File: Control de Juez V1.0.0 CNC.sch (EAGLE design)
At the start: 21 parts, among them Q1 MMBT3904, U1 ATTINY412-SSNSOIC8_SA_SST_MCH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

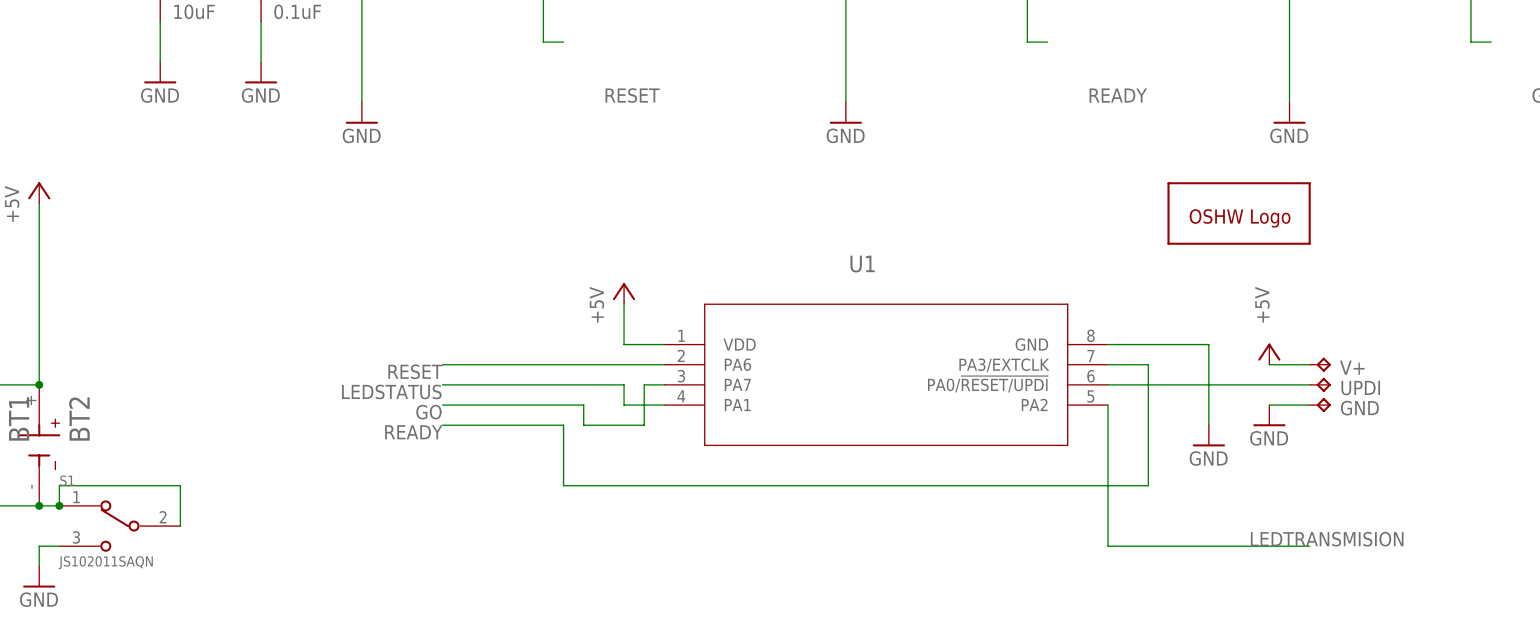
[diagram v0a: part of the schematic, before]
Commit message: Add files via upload
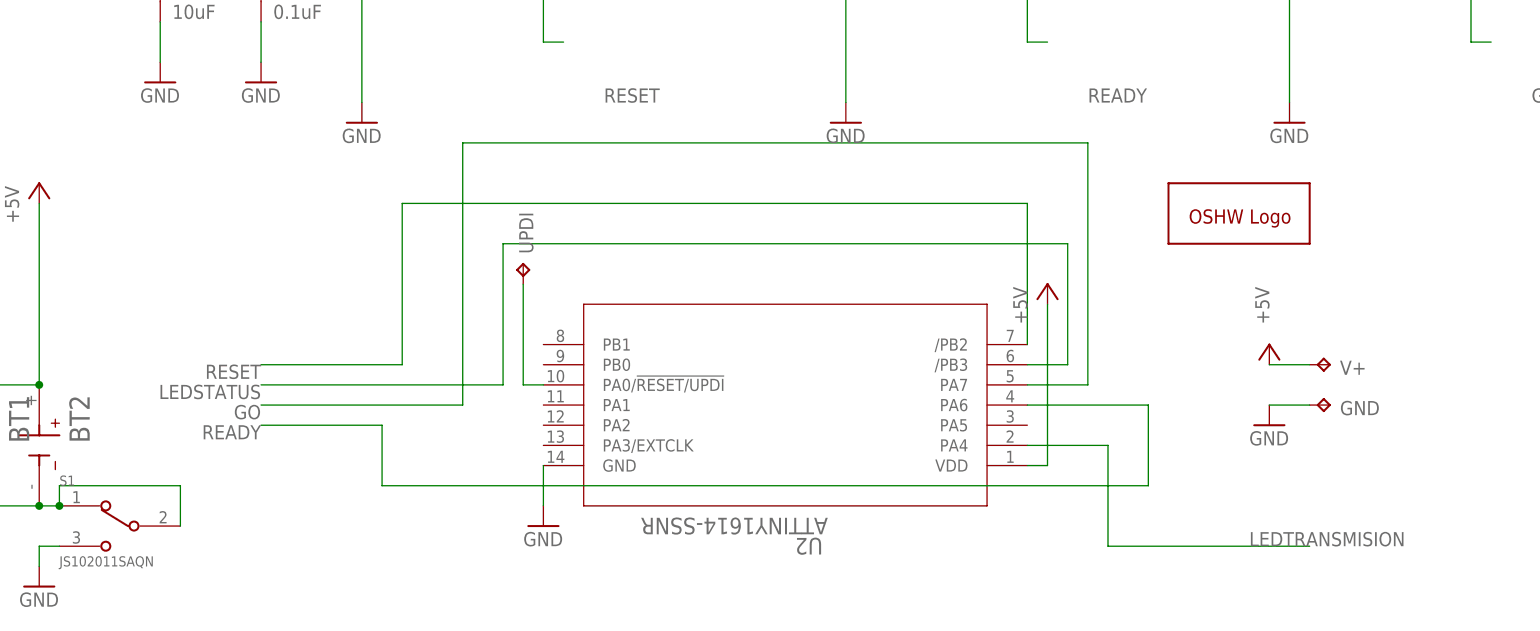
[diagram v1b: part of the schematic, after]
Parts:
- removed U1: ATTINY412-SSNSOIC8_SA_SST_MCH-M, attiny412:ATTINY412-SSNSOIC8_SA_SST_MCH-M
- added U2: ATTINY1614-SSNR, Attiny1614:ATTINY1614-SSNR
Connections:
- removed net N$1: U1.PA0/!RESET/UPDI, UPDI.TP
- new net UPDI: U2.PA0/!RESET/UPDI, UPDI.TP
- net +5V: now also U2.VDD; no longer U1.VDD
- net GND: now also U2.GND; no longer U1.GND
- net GO: now also U2.PA7; no longer U1.PA7
- net LEDSTATUS: now also U2./PB3; no longer U1.PA1
- net LEDTRANSMISION: now also U2.PA4; no longer U1.PA2
- net READY: now also U2.PA6; no longer U1.PA3/EXTCLK
- net RESET: now also U2./PB2; no longer U1.PA6
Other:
- moved on the sheet: UPDI
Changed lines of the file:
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@@
 <part name="GND12" library="supply1" library_urn="urn:adsk.eagle:library:371" deviceset="GND" device=""/>
 <part name="GND13" library="supply1" library_urn="urn:adsk.eagle:library:371" deviceset="GND" device=""/>
-<part name="U1" library="attiny412" deviceset="ATTINY412-SSN" device="SOIC8_SA_SST_MCH-M"/>
 <part name="S1" library="JS102011SAQN" deviceset="JS102011SAQN" device=""/>
 <part name="P+1" library="supply1" library_urn="urn:adsk.eagle:library:371" deviceset="+5V" device=""/>
@@
 <part name="BT1" library="BU2032SM-HD-G" deviceset="BU2032SM-HD-G" device=""/>
 <part name="GOLD_ORB_SM1" library="oshw" deviceset="OSHWLOGO" device="LOGO8MM"/>
+<part name="U2" library="Attiny1614" deviceset="ATTINY1614-SSNR" device=""/>
 </parts>
 <sheets>
@@
 </plain>
 <instances>
-<instance part="GND1" gate="1" x="86.36" y="33.02" smashed="yes">
-<attribute name="VALUE" x="83.82" y="30.48" size="1.778" layer="96"/>
+<instance part="GND1" gate="1" x="2.54" y="22.86" smashed="yes">
+<attribute name="VALUE" x="0" y="20.32" size="1.778" layer="96"/>
 </instance>
 <instance part="C1" gate="G$1" x="-33.02" y="91.44" smashed="yes">
@@
 <attribute name="VALUE" x="93.98" y="71.12" size="1.778" layer="96"/>
 </instance>
-<instance part="U1" gate="A" x="15.24" y="45.72" smashed="yes">
-<attribute name="NAME" x="40.9956" y="54.8386" size="2.0828" layer="95" ratio="6" rot="SR0"/>
-</instance>
 <instance part="S1" gate="G$1" x="-50.8" y="22.86" smashed="yes">
 <attribute name="NAME" x="-58.422909375" y="27.941940625" size="1.270490625" layer="95"/>
 <attribute name="VALUE" x="-58.428559375" y="17.774290625" size="1.27143125" layer="96"/>
 </instance>
-<instance part="P+1" gate="1" x="12.7" y="53.34" smashed="yes">
-<attribute name="VALUE" x="10.16" y="48.26" size="1.778" layer="96" rot="R90"/>
+<instance part="P+1" gate="1" x="66.04" y="53.34" smashed="yes">
+<attribute name="VALUE" x="63.5" y="48.26" size="1.778" layer="96" rot="R90"/>
 </instance>
 <instance part="V+" gate="G$1" x="101.6" y="43.18" smashed="yes" rot="R270">
@@
 <attribute name="TP_SIGNAL_NAME" x="100.33" y="41.91" size="1.778" layer="97" rot="R270"/>
 </instance>
-<instance part="UPDI" gate="G$1" x="101.6" y="40.64" smashed="yes" rot="R270">
-<attribute name="NAME" x="102.87" y="39.37" size="1.778" layer="95"/>
-<attribute name="TP_SIGNAL_NAME" x="100.33" y="39.37" size="1.778" layer="97" rot="R270"/>
+<instance part="UPDI" gate="G$1" x="0" y="55.88" smashed="yes">
+<attribute name="NAME" x="1.27" y="57.15" size="1.778" layer="95" rot="R90"/>
+<attribute name="TP_SIGNAL_NAME" x="1.27" y="54.61" size="1.778" layer="97"/>
 </instance>
 <instance part="GND" gate="G$1" x="101.6" y="38.1" smashed="yes" rot="R270">
@@
 </instance>
 <instance part="GOLD_ORB_SM1" gate="G$1" x="81.28" y="58.42" smashed="yes"/>
+<instance part="U2" gate="A" x="66.04" y="30.48" smashed="yes" rot="R180">
+<attribute name="NAME" x="37.7444" y="21.3614" size="2.0828" layer="95" ratio="6" rot="SR180"/>
+<attribute name="VALUE" x="38.3794" y="23.9014" size="2.0828" layer="96" ratio="6" rot="SR180"/>
+</instance>
 </instances>
 <busses>
@@
 <pinref part="R6" gate="G$1" pin="1"/>
 <wire x1="76.2" y1="160.02" x2="76.2" y2="154.94" width="0.1524" layer="91"/>
-</segment>
-<segment>
-<pinref part="P+1" gate="1" pin="+5V"/>
-<pinref part="U1" gate="A" pin="VDD"/>
-<wire x1="12.7" y1="50.8" x2="12.7" y2="45.72" width="0.1524" layer="91"/>
-<wire x1="12.7" y1="45.72" x2="17.78" y2="45.72" width="0.1524" layer="91"/>
 </segment>
 <segment>
@@
 <junction x="-60.96" y="40.64"/>
 </segment>
+<segment>
+<pinref part="U2" gate="A" pin="VDD"/>
+<pinref part="P+1" gate="1" pin="+5V"/>
+<wire x1="63.5" y1="30.48" x2="66.04" y2="30.48" width="0.1524" layer="91"/>
+<wire x1="66.04" y1="30.48" x2="66.04" y2="50.8" width="0.1524" layer="91"/>
+</segment>
 </net>
 <net name="GND" class="0">
@@
 </segment>
 <segment>
-<pinref part="U1" gate="A" pin="GND"/>
-<pinref part="GND1" gate="1" pin="GND"/>
-<wire x1="73.66" y1="45.72" x2="86.36" y2="45.72" width="0.1524" layer="91"/>
-<wire x1="86.36" y1="45.72" x2="86.36" y2="35.56" width="0.1524" layer="91"/>
-</segment>
-<segment>
 <wire x1="93.98" y1="38.1" x2="99.06" y2="38.1" width="0.1524" layer="91"/>
 <pinref part="GND" gate="G$1" pin="TP"/>
@@
 <wire x1="-60.96" y1="20.32" x2="-60.96" y2="17.78" width="0.1524" layer="91"/>
 </segment>
+<segment>
+<pinref part="U2" gate="A" pin="GND"/>
+<pinref part="GND1" gate="1" pin="GND"/>
+<wire x1="2.54" y1="30.48" x2="2.54" y2="25.4" width="0.1524" layer="91"/>
+</segment>
 </net>
 <net name="N$12" class="0">
@@
 <wire x1="73.66" y1="20.32" x2="99.06" y2="20.32" width="0.1524" layer="91"/>
 <label x="91.44" y="20.32" size="1.778" layer="95"/>
-<pinref part="U1" gate="A" pin="PA2"/>
-<wire x1="73.66" y1="38.1" x2="73.66" y2="20.32" width="0.1524" layer="91"/>
+<pinref part="U2" gate="A" pin="PA4"/>
+<wire x1="73.66" y1="33.02" x2="73.66" y2="20.32" width="0.1524" layer="91"/>
+<wire x1="63.5" y1="33.02" x2="73.66" y2="33.02" width="0.1524" layer="91"/>
 </segment>
 </net>
@@
 <net name="LEDSTATUS" class="0">
 <segment>
-<label x="-10.16" y="40.64" size="1.778" layer="95" rot="R180"/>
-<wire x1="12.7" y1="40.64" x2="-10.16" y2="40.64" width="0.1524" layer="91"/>
-<pinref part="U1" gate="A" pin="PA1"/>
-<wire x1="17.78" y1="38.1" x2="12.7" y2="38.1" width="0.1524" layer="91"/>
-<wire x1="12.7" y1="38.1" x2="12.7" y2="40.64" width="0.1524" layer="91"/>
+<label x="-33.02" y="40.64" size="1.778" layer="95" rot="R180"/>
+<wire x1="-2.54" y1="40.64" x2="-33.02" y2="40.64" width="0.1524" layer="91"/>
+<wire x1="-2.54" y1="40.64" x2="-2.54" y2="58.42" width="0.1524" layer="91"/>
+<wire x1="-2.54" y1="58.42" x2="68.58" y2="58.42" width="0.1524" layer="91"/>
+<pinref part="U2" gate="A" pin="/PB3"/>
+<wire x1="68.58" y1="58.42" x2="68.58" y2="43.18" width="0.1524" layer="91"/>
+<wire x1="68.58" y1="43.18" x2="63.5" y2="43.18" width="0.1524" layer="91"/>
 </segment>
 <segment>
@@
 <net name="READY" class="0">
 <segment>
-<wire x1="5.08" y1="35.56" x2="-10.16" y2="35.56" width="0.1524" layer="91"/>
-<label x="-10.16" y="35.56" size="1.778" layer="95" rot="R180"/>
-<wire x1="5.08" y1="35.56" x2="5.08" y2="27.94" width="0.1524" layer="91"/>
-<wire x1="5.08" y1="27.94" x2="78.74" y2="27.94" width="0.1524" layer="91"/>
-<pinref part="U1" gate="A" pin="PA3/EXTCLK"/>
-<wire x1="78.74" y1="27.94" x2="78.74" y2="43.18" width="0.1524" layer="91"/>
-<wire x1="78.74" y1="43.18" x2="73.66" y2="43.18" width="0.1524" layer="91"/>
+<wire x1="-17.78" y1="35.56" x2="-33.02" y2="35.56" width="0.1524" layer="91"/>
+<label x="-33.02" y="35.56" size="1.778" layer="95" rot="R180"/>
+<wire x1="-17.78" y1="35.56" x2="-17.78" y2="27.94" width="0.1524" layer="91"/>
+<wire x1="-17.78" y1="27.94" x2="78.74" y2="27.94" width="0.1524" layer="91"/>
+<wire x1="78.74" y1="27.94" x2="78.74" y2="38.1" width="0.1524" layer="91"/>
+<pinref part="U2" gate="A" pin="PA6"/>
+<wire x1="63.5" y1="38.1" x2="78.74" y2="38.1" width="0.1524" layer="91"/>
 </segment>
 <segment>
@@
 <net name="GO" class="0">
 <segment>
-<label x="-10.16" y="38.1" size="1.778" layer="95" rot="R180"/>
-<wire x1="7.62" y1="38.1" x2="-10.16" y2="38.1" width="0.1524" layer="91"/>
-<pinref part="U1" gate="A" pin="PA7"/>
-<wire x1="17.78" y1="40.64" x2="15.24" y2="40.64" width="0.1524" layer="91"/>
-<wire x1="15.24" y1="40.64" x2="15.24" y2="35.56" width="0.1524" layer="91"/>
-<wire x1="15.24" y1="35.56" x2="7.62" y2="35.56" width="0.1524" layer="91"/>
-<wire x1="7.62" y1="35.56" x2="7.62" y2="38.1" width="0.1524" layer="91"/>
+<label x="-33.02" y="38.1" size="1.778" layer="95" rot="R180"/>
+<wire x1="-7.62" y1="38.1" x2="-33.02" y2="38.1" width="0.1524" layer="91"/>
+<wire x1="-7.62" y1="38.1" x2="-7.62" y2="71.12" width="0.1524" layer="91"/>
+<wire x1="-7.62" y1="71.12" x2="71.12" y2="71.12" width="0.1524" layer="91"/>
+<wire x1="71.12" y1="71.12" x2="71.12" y2="40.64" width="0.1524" layer="91"/>
+<pinref part="U2" gate="A" pin="PA7"/>
+<wire x1="71.12" y1="40.64" x2="63.5" y2="40.64" width="0.1524" layer="91"/>
 </segment>
 <segment>
@@
 <net name="RESET" class="0">
 <segment>
-<wire x1="17.78" y1="43.18" x2="-10.16" y2="43.18" width="0.1524" layer="91"/>
-<label x="-10.16" y="43.18" size="1.778" layer="95" rot="R180"/>
-<pinref part="U1" gate="A" pin="PA6"/>
+<wire x1="-15.24" y1="43.18" x2="-33.02" y2="43.18" width="0.1524" layer="91"/>
+<label x="-33.02" y="43.18" size="1.778" layer="95" rot="R180"/>
+<wire x1="-15.24" y1="43.18" x2="-15.24" y2="63.5" width="0.1524" layer="91"/>
+<pinref part="U2" gate="A" pin="/PB2"/>
+<wire x1="-15.24" y1="63.5" x2="63.5" y2="63.5" width="0.1524" layer="91"/>
+<wire x1="63.5" y1="63.5" x2="63.5" y2="45.72" width="0.1524" layer="91"/>
 </segment>
 <segment>
@@
 <pinref part="READY" gate="G$1" pin="2"/>
 <wire x1="2.54" y1="96.52" x2="2.54" y2="83.82" width="0.1524" layer="91"/>
-</segment>
-</net>
-<net name="N$1" class="0">
-<segment>
-<pinref part="U1" gate="A" pin="PA0/!RESET/UPDI"/>
-<wire x1="73.66" y1="40.64" x2="99.06" y2="40.64" width="0.1524" layer="91"/>
-<pinref part="UPDI" gate="G$1" pin="TP"/>
 </segment>
 </net>
@@
 </segment>
 </net>
+<net name="UPDI" class="0">
+<segment>
+<pinref part="U2" gate="A" pin="PA0/!RESET/UPDI"/>
+<pinref part="UPDI" gate="G$1" pin="TP"/>
+<wire x1="2.54" y1="40.64" x2="0" y2="40.64" width="0.1524" layer="91"/>
+<wire x1="0" y1="40.64" x2="0" y2="53.34" width="0.1524" layer="91"/>
+</segment>
+</net>
